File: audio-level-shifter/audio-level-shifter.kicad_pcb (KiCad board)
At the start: 2 copper layers, 58 x 18 mm, 11 parts, among them J1 IN, J2 OUT

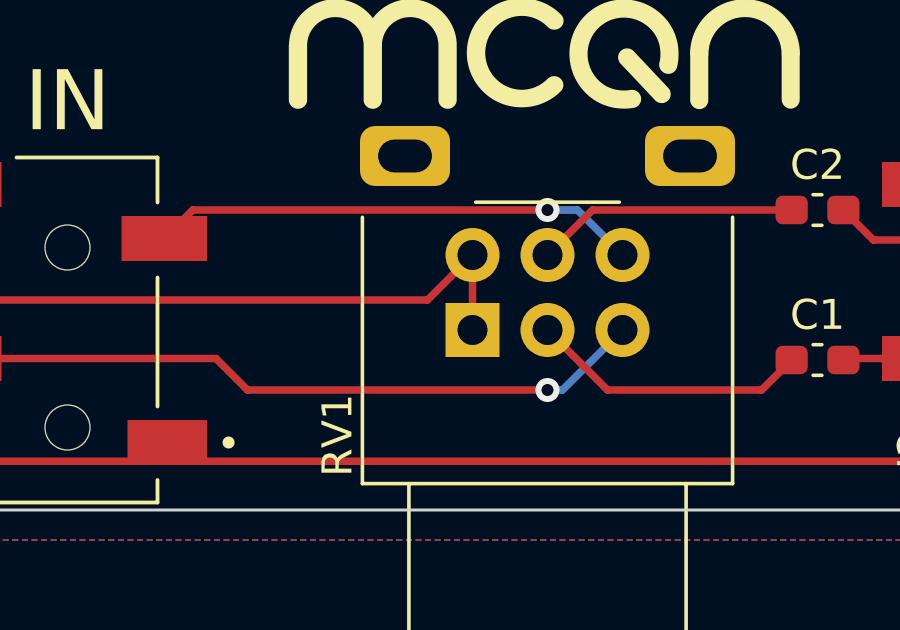
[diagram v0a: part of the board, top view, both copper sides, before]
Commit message: Final tweaks before generating gerbers.
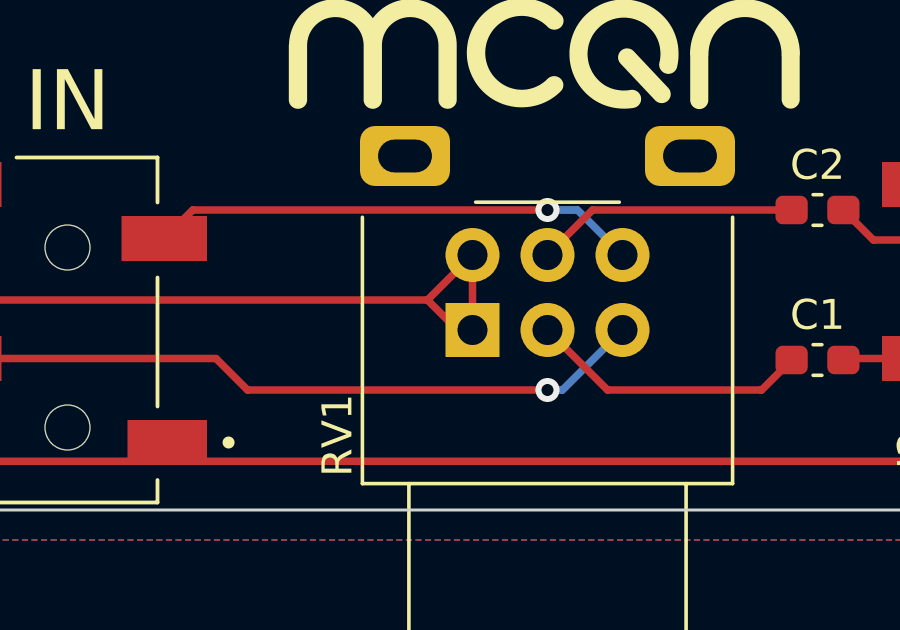
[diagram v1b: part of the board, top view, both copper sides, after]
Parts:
- moved REF** 0.10 mm to (87.8, 91.3)
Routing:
- net GNDA: track 68.1 -> 70.0 mm
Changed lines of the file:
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@@
 			)
 		)
-		(property "Footprint" ""
+		(property "Footprint" "project_libraries:CUI_SJ2-35813B-SMT-TR"
 			(at 0 0 90)
 			(layer "F.Fab")
@@
 			)
 		)
+		(sheetname "Root")
 		(sheetfile "audio-level-shifter.kicad_sch")
 		(attr smd)
@@
 			)
 		)
-		(property "Footprint" ""
+		(property "Footprint" "MountingHole:MountingHole_3.2mm_M3_DIN965"
 			(at 0 0 0)
 			(layer "F.Fab")
@@
 			)
 		)
-		(property "Description" "Mounting Hole without connection"
+		(property "Description" ""
 			(at 0 0 0)
 			(layer "F.Fab")
@@
 			)
 		)
+		(property ki_fp_filters "MountingHole*")
+		(sheetname "Root")
 		(sheetfile "audio-level-shifter.kicad_sch")
 		(attr exclude_from_pos_files)
@@
 			)
 		)
-		(property "Footprint" ""
+		(property "Footprint" "Capacitor_SMD:C_0603_1608Metric_Pad1.08x0.95mm_HandSolder"
 			(at 0 0 180)
 			(layer "F.Fab")
@@
 			)
 		)
-		(property "Description" "Unpolarized capacitor, small symbol"
+		(property "Description" ""
 			(at 0 0 180)
 			(layer "F.Fab")
@@
 			)
 		)
+		(property ki_fp_filters "C_*")
+		(sheetname "Root")
 		(sheetfile "audio-level-shifter.kicad_sch")
 		(attr smd)
@@
 			)
 		)
-		(property "Footprint" ""
+		(property "Footprint" "project_libraries:CUI_SJ2-35813B-SMT-TR"
 			(at 0 0 90)
 			(layer "F.Fab")
@@
 			)
 		)
+		(sheetname "Root")
 		(sheetfile "audio-level-shifter.kicad_sch")
 		(attr smd)
@@
 			)
 		)
-		(property "Footprint" ""
+		(property "Footprint" "Capacitor_SMD:C_0603_1608Metric_Pad1.08x0.95mm_HandSolder"
 			(at 0 0 0)
 			(layer "F.Fab")
@@
 			)
 		)
-		(property "Description" "Unpolarized capacitor, small symbol"
+		(property "Description" ""
 			(at 0 0 0)
 			(layer "F.Fab")
@@
 			)
 		)
+		(property ki_fp_filters "C_*")
+		(sheetname "Root")
 		(sheetfile "audio-level-shifter.kicad_sch")
 		(attr smd)
@@
 			)
 		)
-		(property "Footprint" ""
+		(property "Footprint" "Potentiometer_THT:Potentiometer_Alps_RK09L_Double_Horizontal"
 			(at 0 0 90)
 			(layer "F.Fab")
@@
 			)
 		)
-		(property "Description" "Dual potentiometer"
+		(property "Description" ""
 			(at 0 0 90)
 			(layer "F.Fab")
@@
 			)
 		)
+		(property ki_fp_filters "Potentiometer*")
+		(sheetname "Root")
 		(sheetfile "audio-level-shifter.kicad_sch")
 		(attr through_hole)
@@
 			)
 		)
-		(property "Footprint" ""
+		(property "Footprint" "MountingHole:MountingHole_3.2mm_M3_DIN965"
 			(at 0 0 0)
 			(layer "F.Fab")
@@
 			)
 		)
-		(property "Description" "Mounting Hole without connection"
+		(property "Description" ""
 			(at 0 0 0)
 			(layer "F.Fab")
@@
 			)
 		)
+		(property ki_fp_filters "MountingHole*")
+		(sheetname "Root")
 		(sheetfile "audio-level-shifter.kicad_sch")
 		(attr exclude_from_pos_files)
@@
 			)
 		)
-		(property "Footprint" ""
+		(property "Footprint" "MountingHole:MountingHole_3.2mm_M3_DIN965"
 			(at 0 0 0)
 			(layer "F.Fab")
@@
 			)
 		)
-		(property "Description" "Mounting Hole without connection"
+		(property "Description" ""
 			(at 0 0 0)
 			(layer "F.Fab")
@@
 			)
 		)
+		(property ki_fp_filters "MountingHole*")
+		(sheetname "Root")
 		(sheetfile "audio-level-shifter.kicad_sch")
 		(attr exclude_from_pos_files)
@@
 			)
 		)
-		(property "Footprint" ""
+		(property "Footprint" "MountingHole:MountingHole_3.2mm_M3_DIN965"
 			(at 0 0 0)
 			(layer "F.Fab")
@@
 			)
 		)
-		(property "Description" "Mounting Hole without connection"
+		(property "Description" ""
 			(at 0 0 0)
 			(layer "F.Fab")
@@
 			)
 		)
+		(property ki_fp_filters "MountingHole*")
+		(sheetname "Root")
 		(sheetfile "audio-level-shifter.kicad_sch")
 		(attr exclude_from_pos_files)
@@
 	(footprint "Symbol:OSHW-Logo2_7.3x6mm_SilkScreen"
 		(layer "B.Cu")
-		(at 87.7 91.3 180)
+		(at 87.8 91.3 180)
 		(descr "Open Source Hardware Symbol")
 		(tags "Logo Symbol OSHW")
 		(property "Reference" "REF**"
 			(at 0 0 0)
-			(layer "F.SilkS")
+			(layer "B.SilkS")
 			(hide yes)
 			(effects
@@
 					(thickness 0.15)
 				)
+				(justify mirror)
 			)
 		)
@@
 			)
 		)
-		(property "Footprint" ""
-			(at 0 0 180)
-			(layer "F.Fab")
+		(property "Footprint" "Symbol:OSHW-Logo2_7.3x6mm_SilkScreen"
+			(at 0 0 0)
+			(unlocked yes)
+			(layer "B.Fab")
 			(hide yes)
 			(effects
@@
 					(thickness 0.15)
 				)
+				(justify mirror)
 			)
 		)
 		(property "Datasheet" ""
-			(at 0 0 180)
-			(layer "F.Fab")
+			(at 0 0 0)
+			(unlocked yes)
+			(layer "B.Fab")
 			(hide yes)
 			(effects
@@
 					(thickness 0.15)
 				)
+				(justify mirror)
 			)
 		)
 		(property "Description" ""
-			(at 0 0 180)
-			(layer "F.Fab")
+			(at 0 0 0)
+			(unlocked yes)
+			(layer "B.Fab")
 			(hide yes)
 			(effects
@@
 					(thickness 0.15)
 				)
+				(justify mirror)
 			)
 		)
-		(attr board_only exclude_from_pos_files exclude_from_bom)
+		(attr board_only exclude_from_pos_files exclude_from_bom allow_missing_courtyard)
 		(fp_poly
 			(pts
@@
 			)
 		)
-		(property "Footprint" ""
-			(at 0 0 180)
-			(layer "F.Fab")
+		(property "Footprint" "Symbol:WEEE-Logo_4.2x6mm_SilkScreen"
+			(at 0 0 0)
+			(unlocked yes)
+			(layer "B.Fab")
 			(hide yes)
 			(effects
@@
 					(thickness 0.15)
 				)
+				(justify mirror)
 			)
 		)
 		(property "Datasheet" ""
-			(at 0 0 180)
-			(layer "F.Fab")
+			(at 0 0 0)
+			(unlocked yes)
+			(layer "B.Fab")
 			(hide yes)
 			(effects
@@
 					(thickness 0.15)
 				)
+				(justify mirror)
 			)
 		)
 		(property "Description" ""
-			(at 0 0 180)
-			(layer "F.Fab")
+			(at 0 0 0)
+			(unlocked yes)
+			(layer "B.Fab")
 			(hide yes)
 			(effects
@@
 					(thickness 0.15)
 				)
+				(justify mirror)
 			)
 		)
-		(attr board_only exclude_from_pos_files exclude_from_bom)
+		(attr board_only exclude_from_pos_files exclude_from_bom allow_missing_courtyard)
 		(fp_poly
 			(pts
@@
 	)
 	(segment
+		(start 97 100)
+		(end 96 99)
+		(width 0.25)
+		(layer "F.Cu")
+		(net 5)
+	)
+	(segment
 		(start 97.5 97.5)
 		(end 97.5 100)
@@
 		(width 0.25)
 		(layer "F.Cu")
+		(net 5)
+	)
+	(segment
+		(start 97.5 100)
+		(end 97 100)
+		(width 0.25)
+		(layer "F.Cu")
